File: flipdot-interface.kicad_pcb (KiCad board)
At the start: 4 copper layers, 99.1 x 101.6 mm, 166 parts, among them J1 Conn_02x30_Odd_Even, J2 Conn_02x06_Odd_Even, Q1 BSS123, Q10 BSS123, Q11 BSS123, Q12 BSS84, Q13 BSS84, Q14 BSS84, Q15 BSS123, Q16 BSS123, Q17 BSS123, Q18 BSS84, Q19 BSS84, Q2 BSS84, Q20 BSS84, Q21 BSS123, Q22 BSS123, Q23 BSS123, Q24 BSS84, Q25 BSS84, Q26 BSS84, Q27 BSS123, Q28 BSS123, Q29 BSS123, Q3 BSS123, Q30 BSS84, Q31 BSS84, Q32 BSS84, Q33 BSS123, Q34 BSS123, Q35 BSS123, Q36 BSS84, Q37 BSS84, Q38 BSS84, Q4 BSS123, Q5 BSS123, Q6 BSS84, Q7 BSS84, Q8 BSS84, Q9 BSS123, U1 74HCT595, U10 74LVC1G19, U11 74HCT595, U12 74HCT595, U2 74HCT595, U3 74HCT595, U4 74HCT595, U5 74HCT595, U6 74HCT595, U7 ULN2803A, U8 ULN2803A, U9 ULN2803A

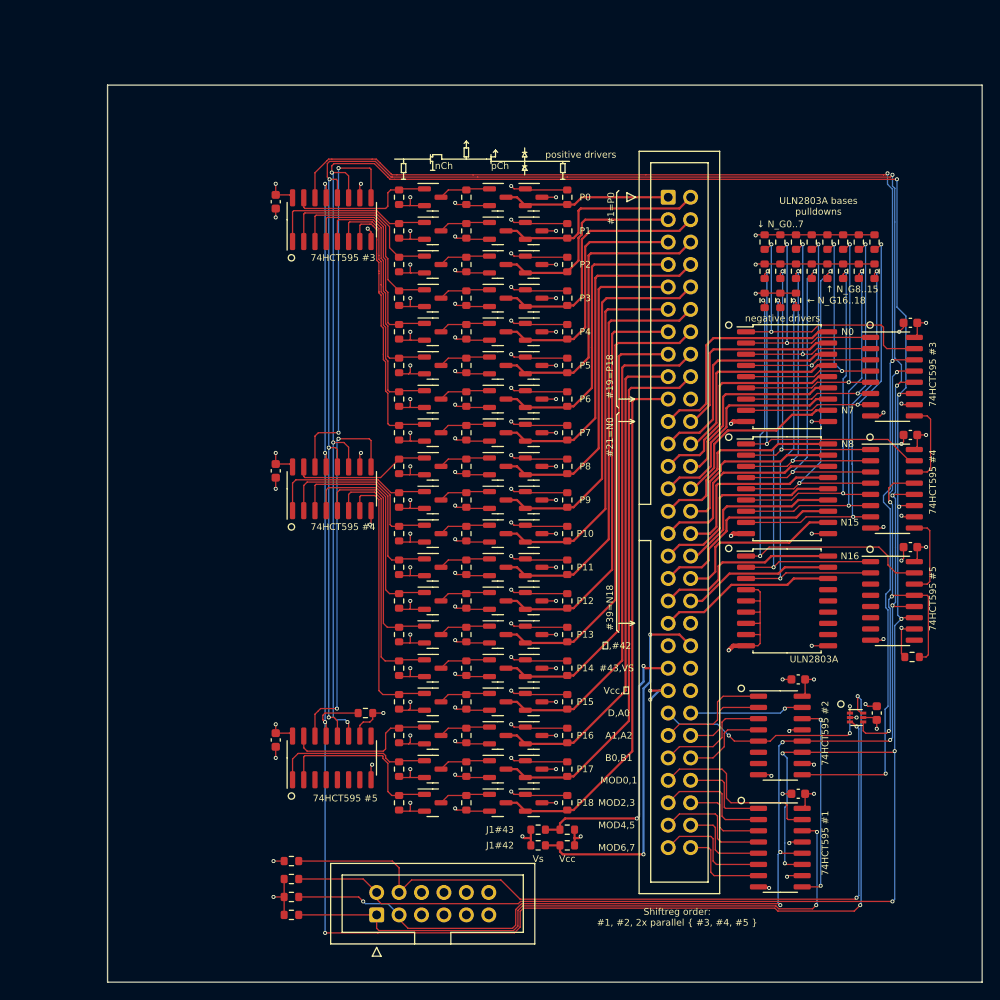
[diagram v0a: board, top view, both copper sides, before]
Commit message: moar woerk
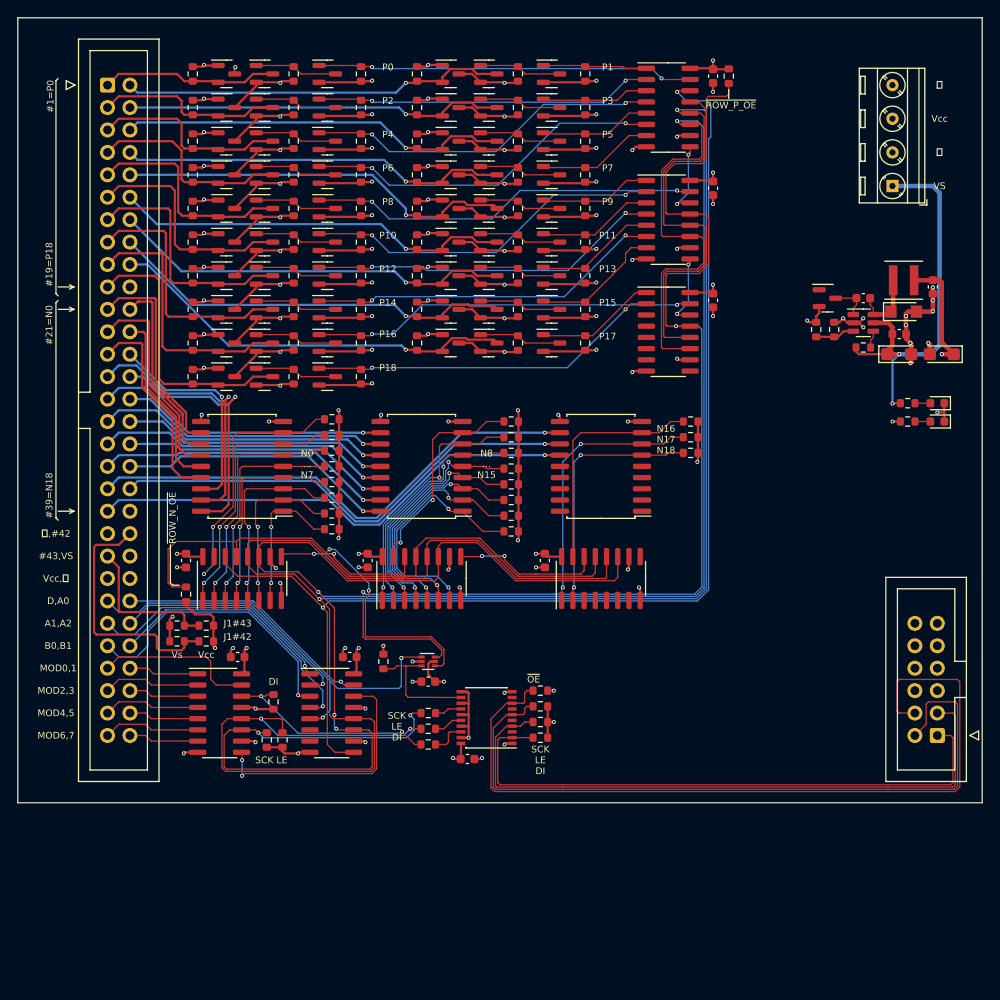
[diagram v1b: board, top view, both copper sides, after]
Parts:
- added C10: 100n, Capacitor_SMD:C_0603_1608Metric, F.Cu at (167.8, 127.1)
- added C11: 100n, Capacitor_SMD:C_0603_1608Metric, F.Cu at (216.7, 79.0)
- added C12: 10u, Capacitor_Tantalum_SMD:CP_EIA-3216-18_Kemet-A, F.Cu at (216.7, 81.3)
- added C13: 100n, Capacitor_SMD:C_0603_1608Metric, F.Cu at (212.6, 74.9)
- added C14: 100n, Capacitor_SMD:C_0603_1608Metric, F.Cu at (220.5, 73.7)
- added C15: 10u, Capacitor_Tantalum_SMD:CP_EIA-3216-18_Kemet-A, F.Cu at (221.5, 81.3)
- added D20: SOT23 A-C-K, Package_TO_SOT_SMD:SOT-23, F.Cu at (208.5, 74.9)
- added D21: SS1P3L, Diode_SMD:D_SMF, F.Cu at (217.2, 76.5)
- added D22: LED, LED_SMD:LED_0603_1608Metric, F.Cu at (221.0, 86.8)
- added D23: LED, LED_SMD:LED_0603_1608Metric, F.Cu at (221.0, 88.9)
- added J3: Screw_Terminal_01x04, TerminalBlock_MetzConnect:TerminalBlock_MetzConnect_Type086_RT03404HBLC_1x04_P3.81mm_Horizontal, F.Cu at (215.9, 62.2)
- added L1: L_Small, Inductor_SMD:L_Coilcraft_XxL4020, F.Cu at (217.2, 72.9)
- added R87: 68R, Resistor_SMD:R_0603_1608Metric, F.Cu at (163.3, 125.5)
- added R88: 68R, Resistor_SMD:R_0603_1608Metric, F.Cu at (163.3, 123.7)
- added R89: 68R, Resistor_SMD:R_0603_1608Metric, F.Cu at (163.3, 121.9)
- added R91: 10k, Resistor_SMD:R_0603_1608Metric, F.Cu at (212.6, 80.5)
- added R92: 150k, Resistor_SMD:R_0603_1608Metric, F.Cu at (207.3, 78.5)
- added R93: 10k, Resistor_SMD:R_0603_1608Metric, F.Cu at (209.3, 78.5)
- added R94: 1k, Resistor_SMD:R_0603_1608Metric, F.Cu at (217.6, 86.8)
- added R95: 1k, Resistor_SMD:R_0603_1608Metric, F.Cu at (217.6, 88.9)
- added R96: 10k, Resistor_SMD:R_0603_1608Metric, F.Cu at (176.0, 119.4)
- added R97: 10k, Resistor_SMD:R_0603_1608Metric, F.Cu at (176.0, 124.7)
- added R98: 10k, Resistor_SMD:R_0603_1608Metric, F.Cu at (176.0, 122.9)
- added R99: 10k, Resistor_SMD:R_0603_1608Metric, F.Cu at (176.0, 121.2)
- added U13: 74HCT244, Package_SO:SSOP-20_4.4x6.5mm_P0.65mm, F.Cu at (169.9, 122.4)
- added U14: LM2734Y, Package_TO_SOT_SMD:TSOT-23-6, F.Cu at (212.6, 77.7)
- moved C1 90.0 mm to (195.6, 49.8)
- moved R58 83.0 mm to (197.4, 49.8), turned to -90 degrees
- moved R59 82.5 mm to (135.9, 108.5), turned to 90 degrees
- moved C4 82.1 mm to (135.9, 104.6), turned to 90 degrees
- moved U4 77.1 mm to (142.2, 106.7), turned to 90 degrees
- moved C5 67.1 mm to (156.5, 104.6), turned to 90 degrees
- moved J2 66.7 mm to (221.0, 124.5), turned to 180 degrees
- moved C9 65.4 mm to (141.7, 115.6)
- moved U12 65.3 mm to (139.7, 121.9)
- moved J1 64.8 mm to (127.0, 50.8)
- moved R77 64.7 mm to (152.4, 88.6), turned to 0 degrees
- moved R12 64.3 mm to (136.7, 83.8)
- moved R75 63.6 mm to (152.4, 90.4), turned to 0 degrees
- moved U7 62.6 mm to (142.2, 94.0), turned to 180 degrees
- moved R73 62.5 mm to (152.4, 92.2), turned to 0 degrees
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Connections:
- J2 pad 1: /DI -> /DI_LV
- J2 pad 2: /SCK -> /SCK_LV
- J2 pad 3: /LE -> /LE_LV
- J2 pad 4: /~{ROW_OE} -> /~{ROW_OE}_LV
- R60 pad 1: /Row Drivers Negative/ROW_N_G0 -> /Row Drivers Negative/ROW_N_G7
- R61 pad 1: /Row Drivers Negative/ROW_N_G8 -> /Row Drivers Negative/ROW_N_G15
- R62 pad 1: /Row Drivers Negative/ROW_N_G16 -> /Row Drivers Negative/ROW_N_G18
- R63 pad 1: /Row Drivers Negative/ROW_N_G1 -> /Row Drivers Negative/ROW_N_G6
- R64 pad 1: /Row Drivers Negative/ROW_N_G9 -> /Row Drivers Negative/ROW_N_G14
- R66 pad 1: /Row Drivers Negative/ROW_N_G2 -> /Row Drivers Negative/ROW_N_G5
- R67 pad 1: /Row Drivers Negative/ROW_N_G10 -> /Row Drivers Negative/ROW_N_G13
- R68 pad 1: /Row Drivers Negative/ROW_N_G18 -> /Row Drivers Negative/ROW_N_G16
- R69 pad 1: /Row Drivers Negative/ROW_N_G3 -> /Row Drivers Negative/ROW_N_G4
- R70 pad 1: /Row Drivers Negative/ROW_N_G11 -> /Row Drivers Negative/ROW_N_G12
- R71 pad 1: /Row Drivers Negative/ROW_N_G4 -> /Row Drivers Negative/ROW_N_G3
- R72 pad 1: /Row Drivers Negative/ROW_N_G12 -> /Row Drivers Negative/ROW_N_G11
- R73 pad 1: /Row Drivers Negative/ROW_N_G5 -> /Row Drivers Negative/ROW_N_G2
- R74 pad 1: /Row Drivers Negative/ROW_N_G13 -> /Row Drivers Negative/ROW_N_G10
- R75 pad 1: /Row Drivers Negative/ROW_N_G6 -> /Row Drivers Negative/ROW_N_G1
- R76 pad 1: /Row Drivers Negative/ROW_N_G14 -> /Row Drivers Negative/ROW_N_G9
- R77 pad 1: /Row Drivers Negative/ROW_N_G7 -> /Row Drivers Negative/ROW_N_G0
- R78 pad 1: /Row Drivers Negative/ROW_N_G15 -> /Row Drivers Negative/ROW_N_G8
- U7 pad 1: /Row Drivers Negative/ROW_N_G0 -> /Row Drivers Negative/ROW_N_G7
- U7 pad 11: /Row Drivers Negative/ROW_N7 -> /Row Drivers Negative/ROW_N0
- U7 pad 12: /Row Drivers Negative/ROW_N6 -> /Row Drivers Negative/ROW_N1
- U7 pad 13: /Row Drivers Negative/ROW_N5 -> /Row Drivers Negative/ROW_N2
- U7 pad 14: /Row Drivers Negative/ROW_N4 -> /Row Drivers Negative/ROW_N3
- U7 pad 15: /Row Drivers Negative/ROW_N3 -> /Row Drivers Negative/ROW_N4
- U7 pad 16: /Row Drivers Negative/ROW_N2 -> /Row Drivers Negative/ROW_N5
- U7 pad 17: /Row Drivers Negative/ROW_N1 -> /Row Drivers Negative/ROW_N6
- U7 pad 18: /Row Drivers Negative/ROW_N0 -> /Row Drivers Negative/ROW_N7
- U7 pad 2: /Row Drivers Negative/ROW_N_G1 -> /Row Drivers Negative/ROW_N_G6
- U7 pad 3: /Row Drivers Negative/ROW_N_G2 -> /Row Drivers Negative/ROW_N_G5
- U7 pad 4: /Row Drivers Negative/ROW_N_G3 -> /Row Drivers Negative/ROW_N_G4
- U7 pad 5: /Row Drivers Negative/ROW_N_G4 -> /Row Drivers Negative/ROW_N_G3
- U7 pad 6: /Row Drivers Negative/ROW_N_G5 -> /Row Drivers Negative/ROW_N_G2
- U7 pad 7: /Row Drivers Negative/ROW_N_G6 -> /Row Drivers Negative/ROW_N_G1
- U7 pad 8: /Row Drivers Negative/ROW_N_G7 -> /Row Drivers Negative/ROW_N_G0
- U8 pad 1: /Row Drivers Negative/ROW_N_G8 -> /Row Drivers Negative/ROW_N_G15
- U8 pad 11: /Row Drivers Negative/ROW_N15 -> /Row Drivers Negative/ROW_N8
- U8 pad 12: /Row Drivers Negative/ROW_N14 -> /Row Drivers Negative/ROW_N9
- U8 pad 13: /Row Drivers Negative/ROW_N13 -> /Row Drivers Negative/ROW_N10
- U8 pad 14: /Row Drivers Negative/ROW_N12 -> /Row Drivers Negative/ROW_N11
- U8 pad 15: /Row Drivers Negative/ROW_N11 -> /Row Drivers Negative/ROW_N12
- U8 pad 16: /Row Drivers Negative/ROW_N10 -> /Row Drivers Negative/ROW_N13
- U8 pad 17: /Row Drivers Negative/ROW_N9 -> /Row Drivers Negative/ROW_N14
- U8 pad 18: /Row Drivers Negative/ROW_N8 -> /Row Drivers Negative/ROW_N15
- U8 pad 2: /Row Drivers Negative/ROW_N_G9 -> /Row Drivers Negative/ROW_N_G14
- U8 pad 3: /Row Drivers Negative/ROW_N_G10 -> /Row Drivers Negative/ROW_N_G13
- U8 pad 4: /Row Drivers Negative/ROW_N_G11 -> /Row Drivers Negative/ROW_N_G12
- U8 pad 5: /Row Drivers Negative/ROW_N_G12 -> /Row Drivers Negative/ROW_N_G11
- U8 pad 6: /Row Drivers Negative/ROW_N_G13 -> /Row Drivers Negative/ROW_N_G10
- U8 pad 7: /Row Drivers Negative/ROW_N_G14 -> /Row Drivers Negative/ROW_N_G9
- U8 pad 8: /Row Drivers Negative/ROW_N_G15 -> /Row Drivers Negative/ROW_N_G8
- U9 pad 1: /Row Drivers Negative/ROW_N_G16 -> (no net)
- U9 pad 11: (no net) -> /Row Drivers Negative/ROW_N16
- U9 pad 12: (no net) -> /Row Drivers Negative/ROW_N17
- U9 pad 13: (no net) -> /Row Drivers Negative/ROW_N18
- U9 pad 16: /Row Drivers Negative/ROW_N18 -> (no net)
- U9 pad 17: /Row Drivers Negative/ROW_N17 -> (no net)
- U9 pad 18: /Row Drivers Negative/ROW_N16 -> (no net)
- U9 pad 2: /Row Drivers Negative/ROW_N_G17 -> (no net)
- U9 pad 3: /Row Drivers Negative/ROW_N_G18 -> (no net)
- U9 pad 4: GND -> (no net)
- U9 pad 5: GND -> (no net)
- U9 pad 6: GND -> /Row Drivers Negative/ROW_N_G18
- U9 pad 7: GND -> /Row Drivers Negative/ROW_N_G17
- U9 pad 8: GND -> /Row Drivers Negative/ROW_N_G16
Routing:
- net VS: track 163.8 -> 263.8 mm, vias 42 -> 26
- net /~{ROW_OE}_LV: track 0.00 -> 92.7 mm
- net /SCK_LV: track 0.00 -> 82.5 mm
- net /~{ROW_OE}: track 88.4 -> 14.1 mm, vias 2 -> 0
- net /LE_LV: track 0.00 -> 72.8 mm
- net /DI_LV: track 0.00 -> 67.7 mm
- net /~{ROW_P_OE}: track 184.1 -> 133.9 mm, vias 6 -> 2
- net /DI: track 72.8 -> 24.2 mm
- net /SCK: track 323.7 -> 276.1 mm, vias 11 -> 6
- net /Row Drivers Negative/ROW_N17: track 17.2 -> 54.6 mm, vias 0 -> 1
- net /Row Drivers Negative/ROW_N16: track 21.1 -> 57.6 mm, vias 0 -> 1
- net /Row Drivers Negative/ROW_N18: track 20.2 -> 56.2 mm, vias 0 -> 1
- net Net-(U1-Pad9): track 43.3 -> 8.59 mm
- net Net-(U2-Pad9): track 42.6 -> 8.34 mm
- net /Row Drivers Positive/ROW_P18: track 61.3 -> 31.1 mm
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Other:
- board size 99.1 x 101.6 mm -> 109.2 x 88.9 mm
- board text added: "DI"
- board text added: "N0 ... N7"
- board text added: "N16 N17 N18"
- board text added: "N8 ... N15"
- board text added: "SCK LE"
- board text added: "SCK LE DI"
- board text added: "VS"
- board text added: "~{OE}"
- board text added: "~{ROW_N_OE}"
- board text added: "~{ROW_P_OE}"
- board text added: "⏚"
- board text removed: "74HCT595 #1"
- board text removed: "74HCT595 #2"
- board text removed: "74HCT595 #3"
- board text removed: "74HCT595 #4"
- board text removed: "74HCT595 #5"
- board text removed: "N0"
- board text removed: "N15"
- board text removed: "N16"
- board text removed: "N7"
- board text removed: "N8"
- board text removed: "Shiftreg order: #1, #2, 2x parallel { #3, #4, #5 }"
- board text removed: "ULN2803A"
- board text removed: "ULN2803A bases pulldowns"
- board text removed: "nCh"
- board text removed: "negative drivers"
- board text removed: "pCh"
- board text removed: "positive drivers"
- board text removed: "← N_G16..18"
- board text removed: "↑ N_G8..15"
- board text removed: "↓ N_G0..7"
